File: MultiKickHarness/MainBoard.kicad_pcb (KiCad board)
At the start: 2 copper layers, 76.2 x 49.5 mm, 27 parts, among them J1 Mortal Kombat 1 Y-Unit, J2 Mortal Kombat 1 T-Unit, J3 Mortal Kombat 2, J4 Mortal Kombat 3, J5 Ultimate Mortal Kombat 3, J6 Mortal Kombat 4, J6D1 P1RUN, J6D2 P2RUN, P0 CONN_01X01, P1 TO CONTROL PANEL

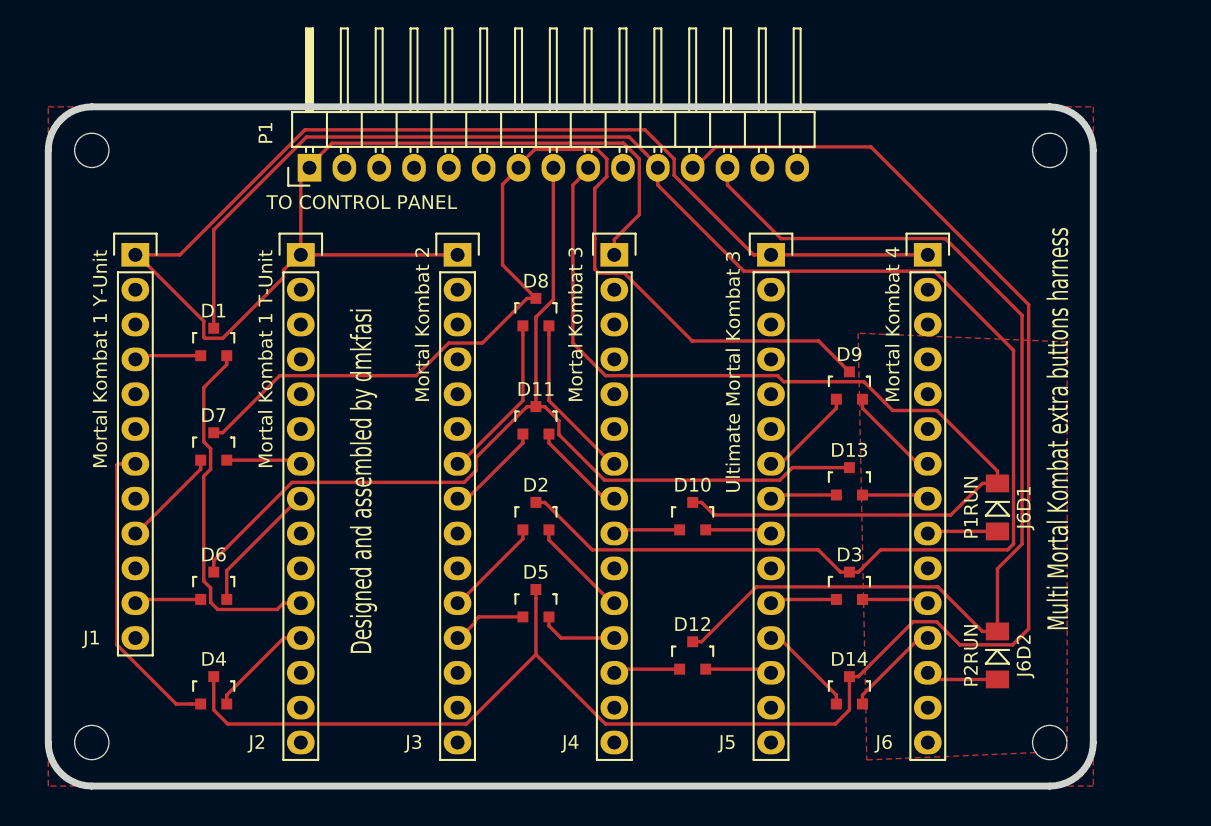
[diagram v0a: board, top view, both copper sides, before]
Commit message: Revision 2
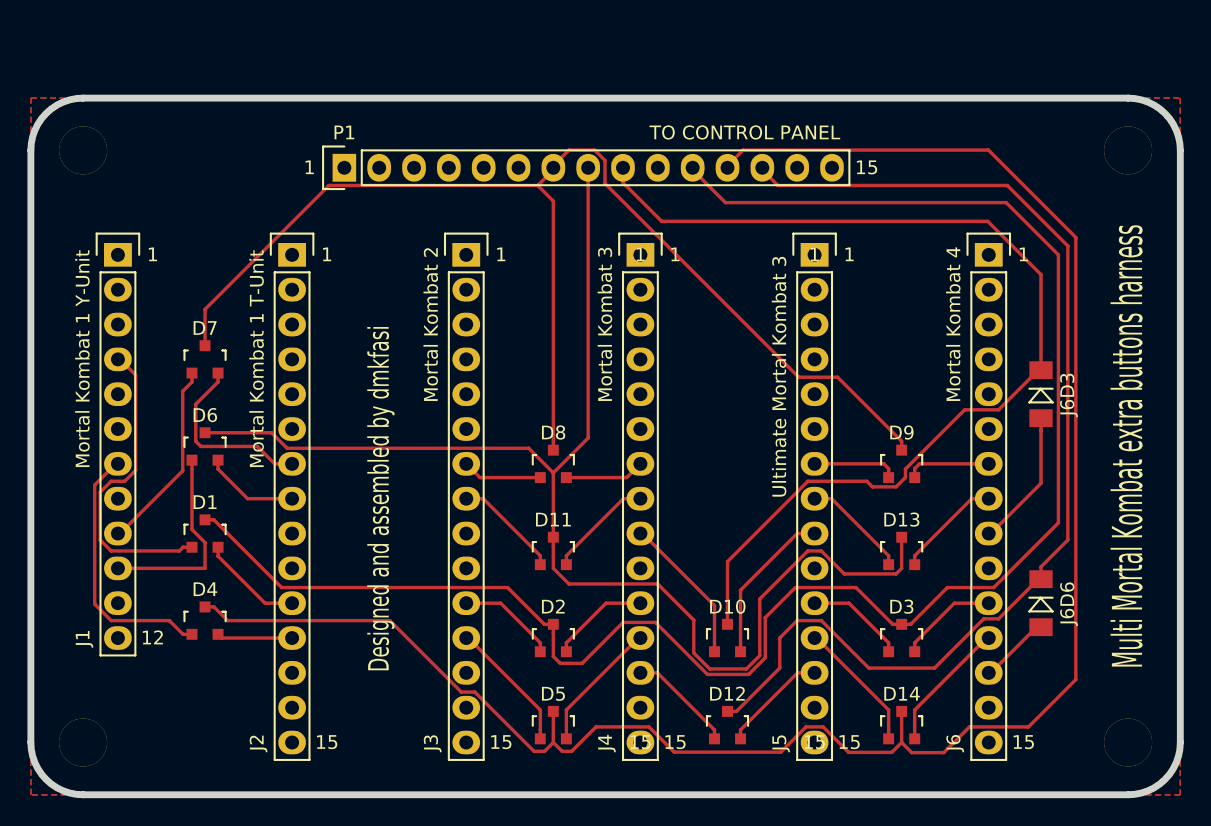
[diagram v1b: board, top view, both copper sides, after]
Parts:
- removed J6D1: P1RUN, Diodes_SMD:MiniMELF_Standard
- removed J6D2: P2RUN, Diodes_SMD:MiniMELF_Standard
- removed the P0 at (85.7, 100.3)
- removed the P0 at (155.6, 100.3)
- removed the P0 at (155.6, 143.5)
- removed the P0 at (85.7, 143.5)
- added J6D3: P1RUN, Diodes_SMD:MiniMELF_Standard, F.Cu at (154.9, 118.1)
- added J6D6: P2RUN, Diodes_SMD:MiniMELF_Standard, F.Cu at (154.9, 133.3)
- added P0: MOUNTING HOLE, Mounting_Holes:MountingHole_3-5mm, F.Cu at (161.3, 100.3)
- added P0: MOUNTING HOLE, Mounting_Holes:MountingHole_3-5mm, F.Cu at (161.3, 143.5)
- added P0: MOUNTING HOLE, Mounting_Holes:MountingHole_3-5mm, F.Cu at (85.1, 143.5)
- added P0: MOUNTING HOLE, Mounting_Holes:MountingHole_3-5mm, F.Cu at (85.1, 100.3)
- added REF**: Symbol_OSHW-Logo_SilkScreen, Symbols:Symbol_OSHW-Logo_SilkScreen, B.Cu at (118.1, 114.3)
- D14: value P2LP -> P2LK
- P1: footprint Pin_Headers:Pin_Header_Angled_1x15 -> Pin_Headers:Pin_Header_Straight_1x15
- moved D1 14.0 mm to (94.0, 128.3)
- moved D8 11.1 mm to (119.4, 123.2)
- moved D6 10.2 mm to (94.0, 121.9)
- moved D11 9.61 mm to (119.4, 129.5)
- moved D10 9.25 mm to (132.1, 135.9)
- moved D5 8.98 mm to (119.4, 142.2)
- moved D2 8.98 mm to (119.4, 135.9)
- moved D9 6.87 mm to (144.8, 123.2)
- moved D7 6.38 mm to (94.0, 115.6)
- moved D13 6.35 mm to (144.8, 129.5)
- moved D12 5.68 mm to (132.1, 142.2)
- moved D3 5.39 mm to (144.8, 135.9)
- moved D4 5.12 mm to (94.0, 134.6)
- moved D14 4.58 mm to (144.8, 142.2)
- moved J6 4.44 mm to (151.1, 108.0)
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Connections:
- net Net-(D1-Pad3) renamed /P2-LP
- net Net-(D10-Pad3) renamed /P1-RUN
- net Net-(D11-Pad3) renamed /P1-LK
- net Net-(D12-Pad3) renamed /P2-RUN
- net Net-(D14-Pad3) renamed /P2-LK
- net Net-(D7-Pad3) renamed /P1-LP
- J1 pad 10: (no net) -> Net-(D6-Pad1)
- J1 pad 11: Net-(D6-Pad1) -> (no net)
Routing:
- net /GND: track 135.3 -> 0.00 mm
- net /P1-LK: track 73.5 -> 95.8 mm
- net Net-(D1-Pad2): track 26.3 -> 7.47 mm
- net Net-(D1-Pad1): track 4.88 -> 22.6 mm
- net /P1-LP: track 75.9 -> 88.6 mm
- net Net-(D6-Pad1): track 4.88 -> 14.6 mm
- net /P2-LK: track 130.7 -> 139.7 mm
- net Net-(D7-Pad2): track 5.51 -> 13.4 mm
- net Net-(D10-Pad2): track 4.88 -> 11.6 mm
- net Net-(D7-Pad1): track 7.36 -> 14.0 mm
- net Net-(D8-Pad2): track 12.1 -> 5.81 mm
- net Net-(D8-Pad1): track 12.1 -> 5.81 mm
- net Net-(D10-Pad1): track 4.88 -> 10.9 mm
- net /P2-RUN: track 75.7 -> 80.8 mm
- net Net-(J6-Pad9): track 5.14 -> 10.1 mm
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- added copper zone on B.Cu, net /GND
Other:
- board size 76.2 x 49.5 mm -> 83.8 x 50.8 mm
- net class Default: clearance 0.2 -> 0.15
- rule trace_clearance: 0.2 -> 0.15
- board text added: "1"
- board text added: "12"
- board text added: "15"
- board text added: "Rev.2"
